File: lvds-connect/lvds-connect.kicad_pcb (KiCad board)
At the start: 2 copper layers, 7.7 x 30.5 mm, 2 parts, among them J1 Conn_02x15_Odd_Even, J2 Conn_01x22

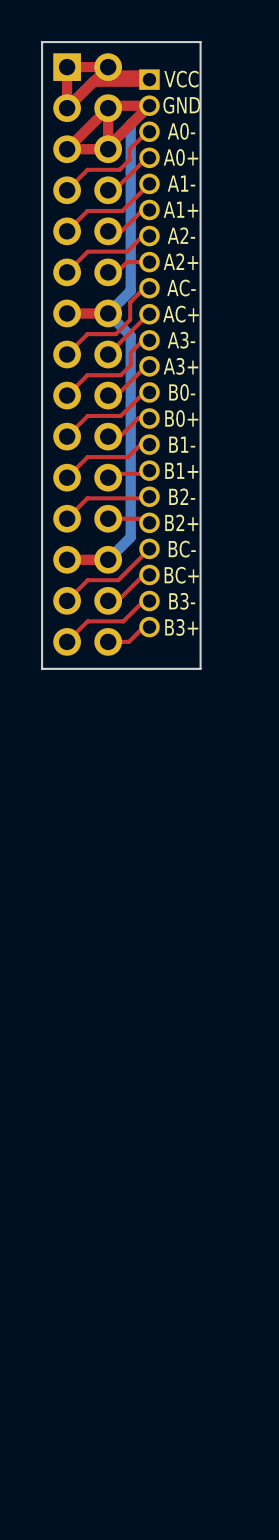
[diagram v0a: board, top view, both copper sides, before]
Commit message: 도면 태그 기입
Signed-off-by: Ju, Gyeong-min <jcmh74@gmail.com>
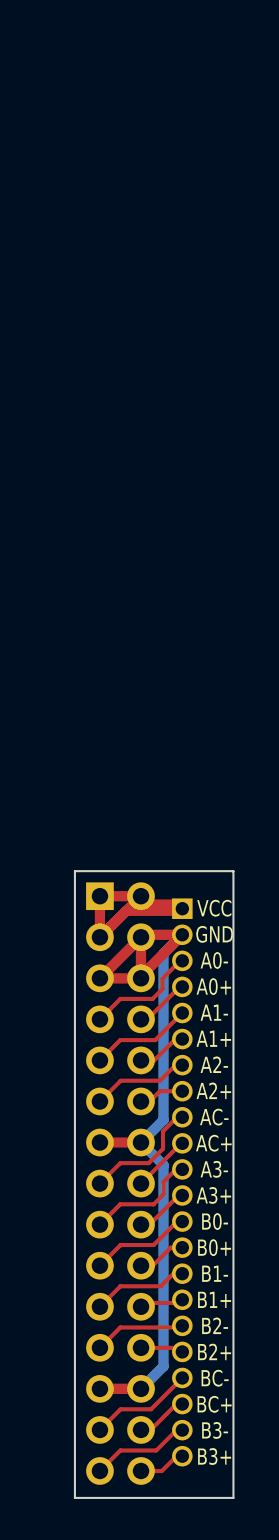
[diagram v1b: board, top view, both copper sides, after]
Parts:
- moved J1 40.4 mm to (141.4, 83.1)
- moved J2 40.4 mm to (145.4, 83.7)
